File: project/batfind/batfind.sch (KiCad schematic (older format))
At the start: 0 parts

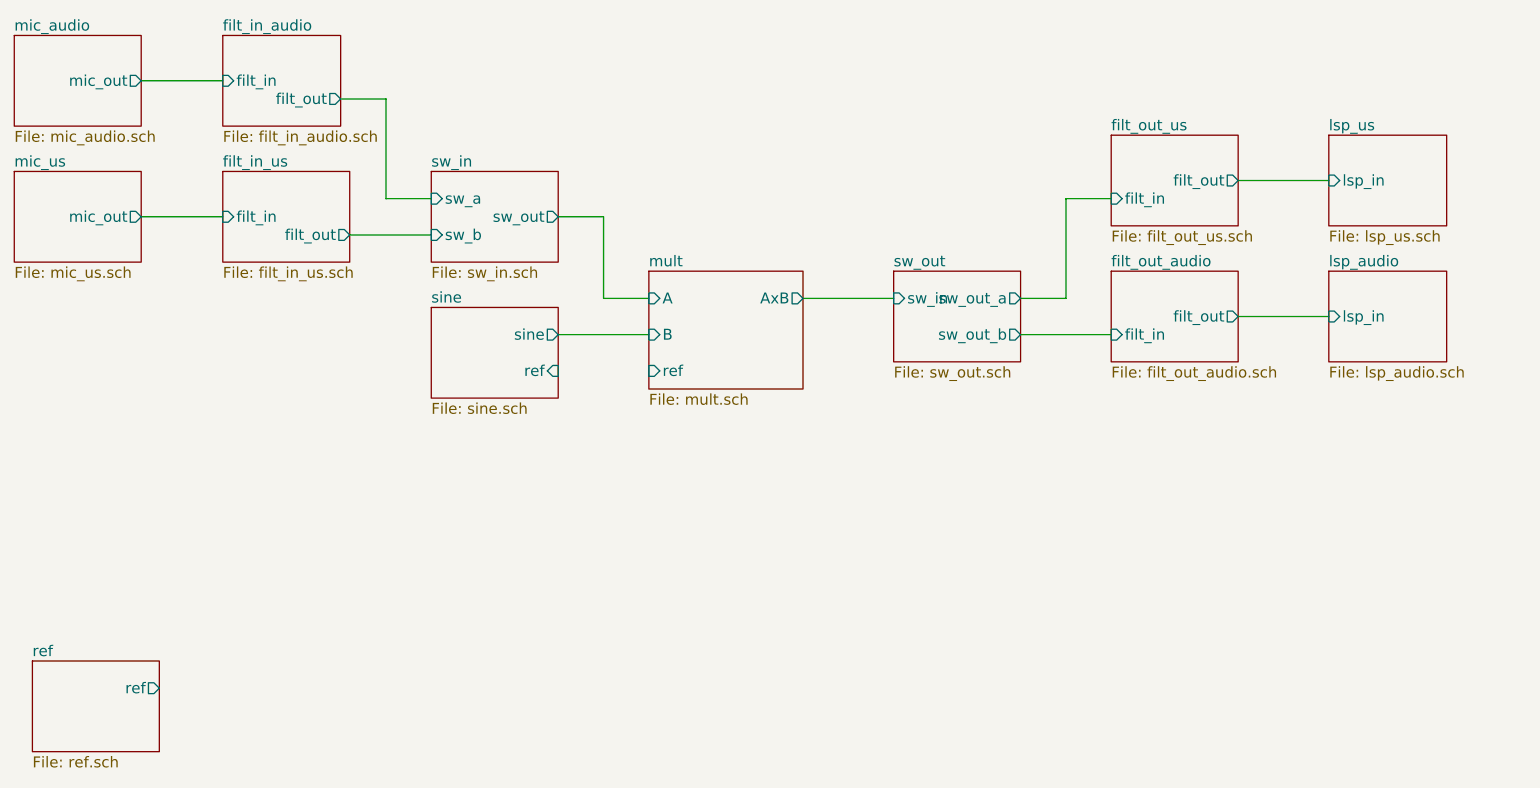
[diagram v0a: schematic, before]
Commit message: Schematic updated
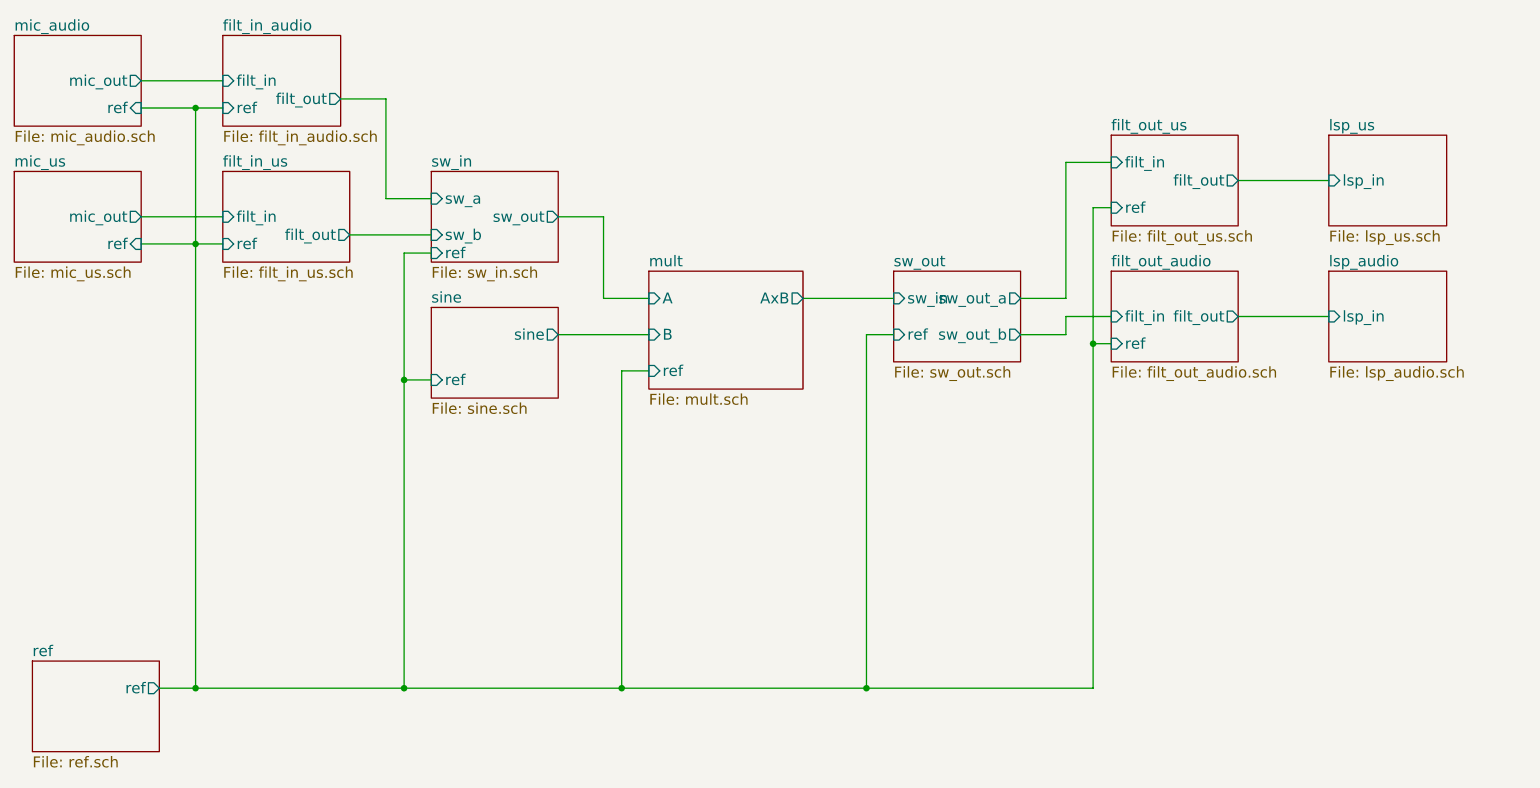
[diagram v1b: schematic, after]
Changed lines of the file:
@@
 F0 "sine" 60
 F1 "sine.sch" 60
-F2 "ref" I R 4750 3700 60
+F2 "ref" I L 4050 3750 60
 F3 "sine" O R 4750 3500 60
 $EndSheet
@@
 F3 "sw_a" I L 4050 2750 60
 F4 "sw_b" I L 4050 2950 60
+F5 "ref" I L 4050 3050 60
 $EndSheet
 $Sheet
@@
 F3 "sw_out_a" O R 7300 3300 60
 F4 "sw_out_b" O R 7300 3500 60
+F5 "ref" I L 6600 3500 60
 $EndSheet
 $Sheet
@@
 F0 "filt_out_audio" 60
 F1 "filt_out_audio.sch" 60
-F2 "filt_in" I L 7800 3500 60
+F2 "filt_in" I L 7800 3400 60
 F3 "filt_out" O R 8500 3400 60
+F4 "ref" I L 7800 3550 60
 $EndSheet
 $Sheet
@@
 F0 "filt_out_us" 60
 F1 "filt_out_us.sch" 60
-F2 "filt_in" I L 7800 2750 60
+F2 "filt_in" I L 7800 2550 60
 F3 "filt_out" O R 8500 2650 60
+F4 "ref" I L 7800 2800 60
 $EndSheet
 $Sheet
@@
 F2 "filt_in" I L 2900 2850 60
 F3 "filt_out" O R 3600 2950 60
+F4 "ref" I L 2900 3000 60
 $EndSheet
 $Sheet
@@
 F2 "filt_in" I L 2900 2100 60
 F3 "filt_out" O R 3550 2200 60
+F4 "ref" I L 2900 2250 60
 $EndSheet
 $Sheet
@@
 F1 "mic_us.sch" 60
 F2 "mic_out" O R 2450 2850 60
+F3 "ref" I R 2450 3000 60
 $EndSheet
 $Sheet
@@
 F1 "mic_audio.sch" 60
 F2 "mic_out" O R 2450 2100 60
+F3 "ref" I R 2450 2250 60
 $EndSheet
 $Sheet
@@
 	6100 3300 6600 3300
 Wire Wire Line
-	7300 3500 7800 3500
+	7550 3300 7300 3300
 Wire Wire Line
-	7300 3300 7550 3300
-Wire Wire Line
-	7550 3300 7550 2750
-Wire Wire Line
-	7550 2750 7800 2750
+	7550 2550 7550 3300
 Wire Wire Line
 	8500 2650 9000 2650
 Wire Wire Line
 	8500 3400 9000 3400
+Wire Wire Line
+	7300 3500 7550 3500
+Wire Wire Line
+	7550 3500 7550 3400
+Wire Wire Line
+	7550 3400 7800 3400
+Wire Wire Line
+	7550 2550 7800 2550
+Wire Wire Line
+	2550 5450 7700 5450
+Wire Wire Line
+	6450 5450 6450 3500
+Wire Wire Line
+	6450 3500 6600 3500
+Wire Wire Line
+	5250 3700 5100 3700
+Wire Wire Line
+	5100 3700 5100 5450
+Connection ~ 5100 5450
+Wire Wire Line
+	7800 2800 7700 2800
+Wire Wire Line
+	7700 2800 7700 5450
+Connection ~ 6450 5450
+Wire Wire Line
+	7800 3550 7700 3550
+Connection ~ 7700 3550
+Wire Wire Line
+	4050 3050 3900 3050
+Wire Wire Line
+	3900 3050 3900 5450
+Connection ~ 3900 5450
+Wire Wire Line
+	4050 3750 3900 3750
+Connection ~ 3900 3750
+Wire Wire Line
+	2450 2250 2900 2250
+Wire Wire Line
+	2750 2250 2750 5450
+Connection ~ 2750 5450
+Wire Wire Line
+	2450 3000 2900 3000
+Connection ~ 2750 3000
+Connection ~ 2750 2250
 $EndSCHEMATC
